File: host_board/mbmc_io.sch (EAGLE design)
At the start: 73 parts, among them IC1 ULN2803, IC2 DIP Socket, IC3 REF02 5 VOLTS, IC4 5 VOLTS, IC5 12 VOLTS, IC6 3.3 VOLTS, J1 1-1586043-4, J2 1586044-4

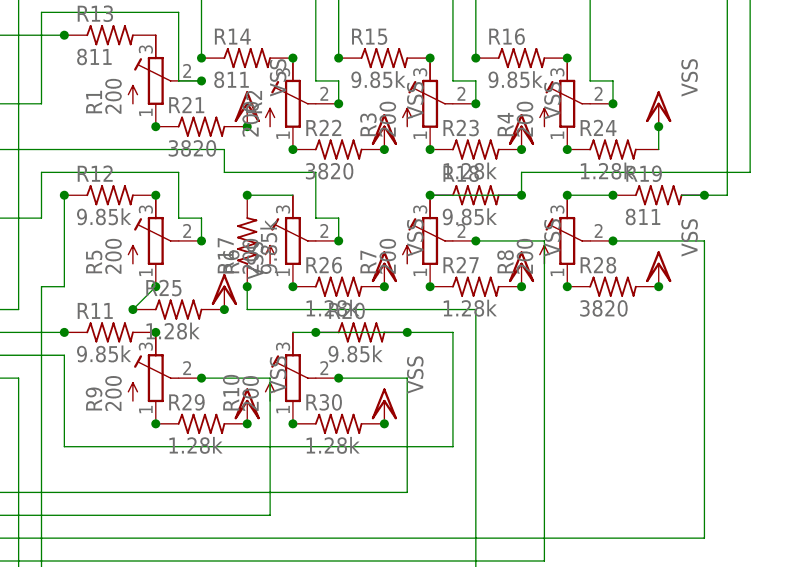
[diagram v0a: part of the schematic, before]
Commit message: up
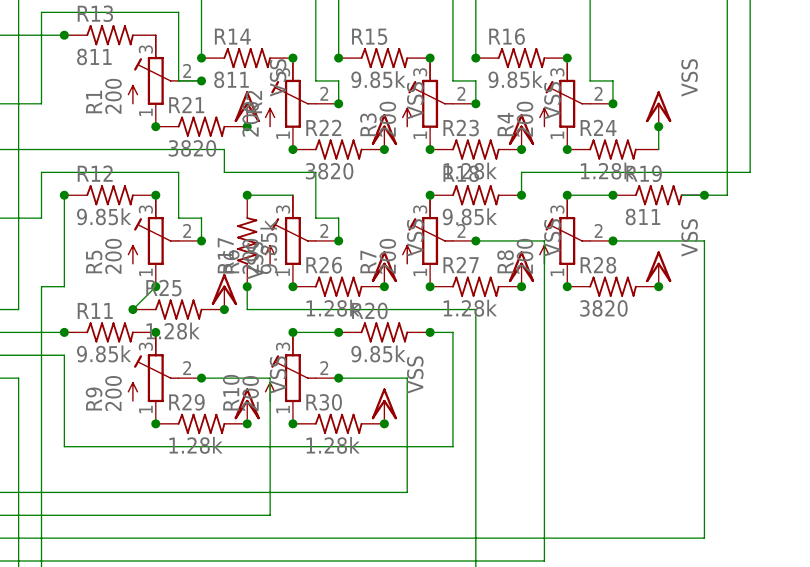
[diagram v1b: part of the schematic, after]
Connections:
- new net N$83: R10.E, R20.1
- new net N$88: R18.1, R7.E
- net N$71: no longer R10.E, R20.1
- net N$8: no longer R18.1, R7.E
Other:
- moved on the sheet: R20
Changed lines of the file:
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@@
 <class number="0" name="default" width="0" drill="0">
 </class>
-<class number="1" name="i-lines" width="0.5" drill="0">
+<class number="1" name="i-lines" width="0.4" drill="0">
 </class>
 </classes>
@@
 <attribute name="VALUE" x="95.25" y="72.898" size="1.778" layer="96"/>
 </instance>
-<instance part="R20" gate="G$1" x="66.04" y="60.96" smashed="yes">
-<attribute name="NAME" x="62.23" y="62.4586" size="1.778" layer="95"/>
-<attribute name="VALUE" x="62.23" y="57.658" size="1.778" layer="96"/>
+<instance part="R20" gate="G$1" x="68.58" y="60.96" smashed="yes">
+<attribute name="NAME" x="64.77" y="62.4586" size="1.778" layer="95"/>
+<attribute name="VALUE" x="64.77" y="57.658" size="1.778" layer="96"/>
 </instance>
 <instance part="R21" gate="G$1" x="48.26" y="83.82" smashed="yes">
@@
 <net name="N$8" class="0">
 <segment>
-<pinref part="R7" gate="G$1" pin="E"/>
 <pinref part="R18" gate="G$1" pin="2"/>
-<wire x1="83.82" y1="76.2" x2="73.66" y2="76.2" width="0.1524" layer="91"/>
-<pinref part="R18" gate="G$1" pin="1"/>
-<junction x="73.66" y="76.2"/>
 <wire x1="83.82" y1="76.2" x2="83.82" y2="78.74" width="0.1524" layer="91"/>
 <wire x1="83.82" y1="78.74" x2="109.22" y2="78.74" width="0.1524" layer="91"/>
@@
 <wire x1="33.02" y1="48.26" x2="76.2" y2="48.26" width="0.1524" layer="91"/>
 <wire x1="76.2" y1="48.26" x2="76.2" y2="60.96" width="0.1524" layer="91"/>
-<pinref part="R10" gate="G$1" pin="E"/>
 <pinref part="R20" gate="G$1" pin="2"/>
-<wire x1="71.12" y1="60.96" x2="60.96" y2="60.96" width="0.1524" layer="91"/>
-<pinref part="R20" gate="G$1" pin="1"/>
-<wire x1="60.96" y1="60.96" x2="58.42" y2="60.96" width="0.1524" layer="91"/>
-<junction x="60.96" y="60.96"/>
-<wire x1="76.2" y1="60.96" x2="71.12" y2="60.96" width="0.1524" layer="91"/>
-<junction x="71.12" y="60.96"/>
+<wire x1="76.2" y1="60.96" x2="73.66" y2="60.96" width="0.1524" layer="91"/>
 <junction x="-48.26" y="81.28"/>
+<junction x="73.66" y="60.96"/>
 </segment>
 </net>
@@
 </segment>
 </net>
+<net name="N$83" class="0">
+<segment>
+<pinref part="R10" gate="G$1" pin="E"/>
+<pinref part="R20" gate="G$1" pin="1"/>
+<wire x1="58.42" y1="60.96" x2="63.5" y2="60.96" width="0.1524" layer="91"/>
+<junction x="58.42" y="60.96"/>
+<junction x="63.5" y="60.96"/>
+</segment>
+</net>
+<net name="N$88" class="0">
+<segment>
+<pinref part="R7" gate="G$1" pin="E"/>
+<pinref part="R18" gate="G$1" pin="1"/>
+<junction x="73.66" y="76.2"/>
+</segment>
+</net>
